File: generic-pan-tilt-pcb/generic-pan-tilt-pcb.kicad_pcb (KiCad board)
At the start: 2 copper layers, 104 x 57 mm, 89 parts, among them J1 B4P-VH-FB-B, J10 USB4105-GF-A, J11 Conn_01x08, J12 Conn_01x08, J13 Conn_01x05, J2 NC5MAV, J3 NC5FAV, J5 BM03B-SRSS-TBT, J7 BM03B-SRSS-TBT, J8 B12B-PH-SM4-TBT, J9 B12B-PH-SM4-TBT, SW1 PTS 647 SK70 SMTR2 LFS, SW2 PTS 647 SK70 SMTR2 LFS, SW3 219-12LPST, U1 RP2040, U2 W25Q128JVS, U3 AP63203WU, U4 ISO1450DW, U5 MCP23017_SO, U6 LIS3DH, Y1 ABM8-272-T3

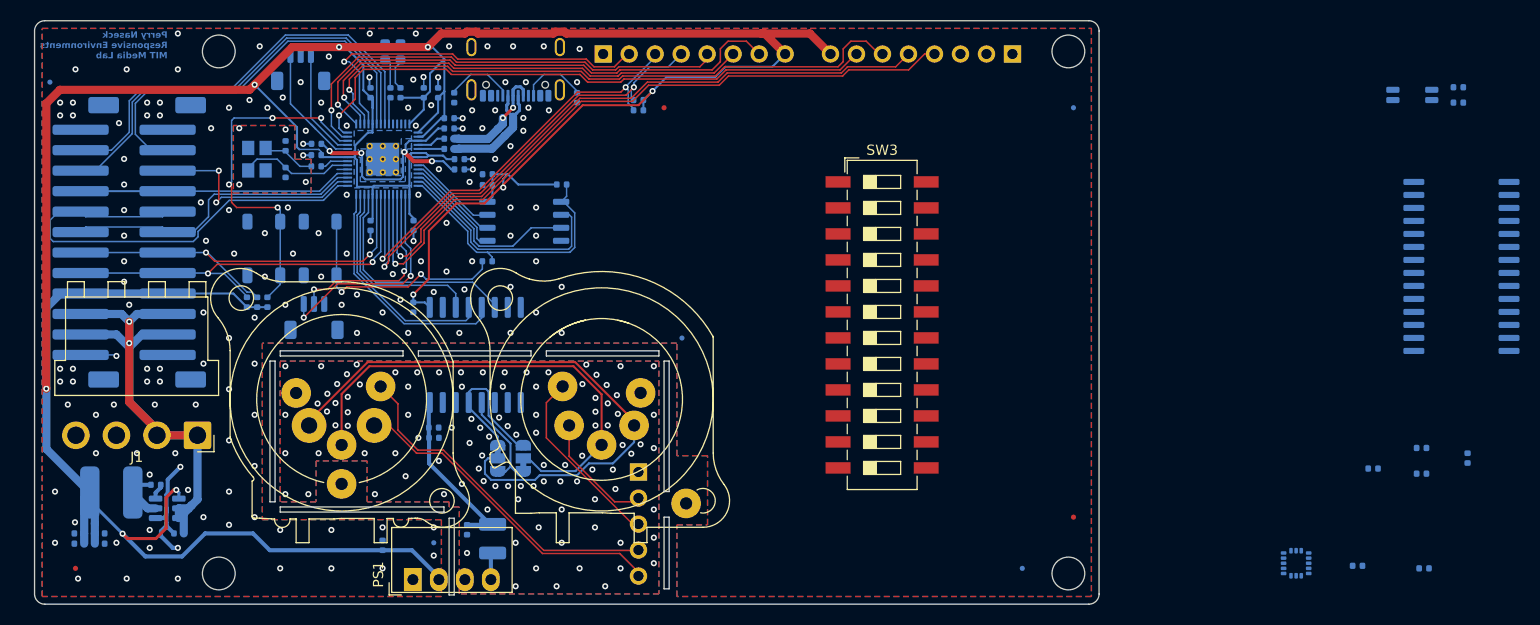
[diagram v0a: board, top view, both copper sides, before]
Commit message: routing done, add oshw and license
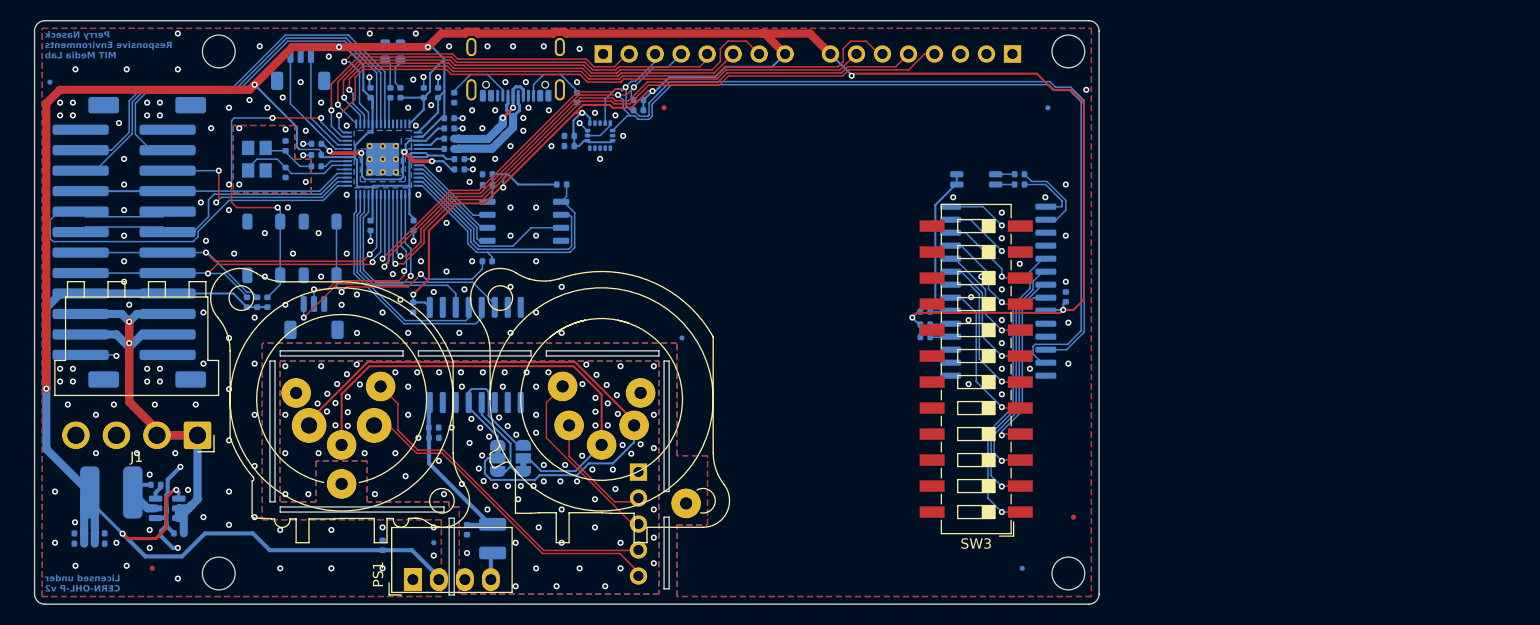
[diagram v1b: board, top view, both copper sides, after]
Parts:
- added SYM1: Logo_Open_Hardware_Small, Symbol:OSHW-Logo2_7.3x6mm_SilkScreen, B.Cu at (107.5, 119.8)
- moved C30 93.1 mm to (133.2, 78.8)
- moved C29 87.7 mm to (133.2, 77.8)
- moved U6 79.8 mm to (136.2, 77.7), turned to -90 degrees
- moved R17 50.6 mm to (168.0, 96.2), turned to 0 degrees
- moved R16 50.3 mm to (168.0, 94.9), turned to 0 degrees
- moved R15 45.6 mm to (168.0, 97.4), turned to 0 degrees
- moved U5 45.3 mm to (175.2, 92.9), turned to 180 degrees
- moved R19 43.7 mm to (177.2, 81.5)
- moved R18 43.6 mm to (177.2, 82.5)
- moved D3 43.4 mm to (173.0, 82.0)
- moved C28 42.3 mm to (181.8, 93.5), turned to 90 degrees
- moved SW3 10.2 mm to (173.0, 100.5), turned to 180 degrees
- moved FID6 7.50 mm to (92.5, 120.0)
- moved FID2 2.50 mm to (180.0, 75.0)
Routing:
- net +3V3: track 362.2 -> 457.3 mm, vias 9 -> 13
- net /I2C0_SDA: track 47.8 -> 129.4 mm, vias 2 -> 3
- net /I2C0_SCL: track 44.1 -> 122.6 mm
- net /generic-pan-tilt-pcb_hid/DIP0: track 0.00 -> 29.6 mm, vias 0 -> 1
- net /generic-pan-tilt-pcb_hid/DIP1: track 0.00 -> 25.6 mm, vias 0 -> 1
- net /generic-pan-tilt-pcb_hid/DIP2: track 0.00 -> 21.6 mm, vias 0 -> 1
- net /generic-pan-tilt-pcb_hid/DIP3: track 0.00 -> 17.8 mm, vias 0 -> 1
- net /generic-pan-tilt-pcb_hid/DIP4: track 0.00 -> 15.2 mm, vias 0 -> 1
- net /generic-pan-tilt-pcb_hid/DIP5: track 0.00 -> 14.5 mm, vias 0 -> 1
- net /generic-pan-tilt-pcb_hid/DIP6: track 0.00 -> 12.7 mm, vias 0 -> 1
- net /generic-pan-tilt-pcb_hid/DIP7: track 0.00 -> 11.1 mm, vias 0 -> 1
- net /generic-pan-tilt-pcb_hid/DIP8: track 0.00 -> 10.1 mm, vias 0 -> 1
- net /generic-pan-tilt-pcb_hid/DIP9: track 0.00 -> 9.08 mm, vias 0 -> 1
- net /generic-pan-tilt-pcb_hid/LED1_G: track 0.00 -> 8.39 mm
- net /generic-pan-tilt-pcb_hid/DIP10: track 0.00 -> 6.27 mm, vias 0 -> 1
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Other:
- board text added: "Licensed under CERN-OHL-P v2"
- board text added: "https://github.com/mitmedialab/generic-pan-tilt-pcb/"
